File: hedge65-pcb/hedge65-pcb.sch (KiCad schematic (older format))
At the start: 164 parts, among them J1 USB_C_Receptacle_USB2.0, SW1 SW_PUSH, U1 ATmega32U4-AU, Y1 16MHz

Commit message: schematic done
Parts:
- C1, C2, C3, C4, C5, C6, C7: footprint (none) -> Capacitor_SMD:C_0805_2012Metric
- D1, D10, D11, D12, D13, D14, D15, D16, D17, D18, D19, D2, D20, D21, D22, D23, D24, D25, D26, D27, D28, D29, D3, D30, D31, D32, D33, D34, D35, D36, D37, D38, D39, D4, D40, D41, D42, D43, D44, D45, D46, D47, D48, D49, D5, D50, D51, D52, D53, D54, D55, D56, D57, D58, D59, D6, D60, D61, D62, D63, D64, D65, D66, D67, D68, D69, D7, D70, D71, D72, D73, D8, D9: footprint (none) -> Diode_SMD:D_SOD-123
- F1: footprint (none) -> Fuse:Fuse_1206_3216Metric
- J1: footprint (none) -> Type-C:HRO-TYPE-C-31-M-12-HandSoldering
- Y1: footprint (none) -> Crystal:Crystal_SMD_3225-4Pin_3.2x2.5mm

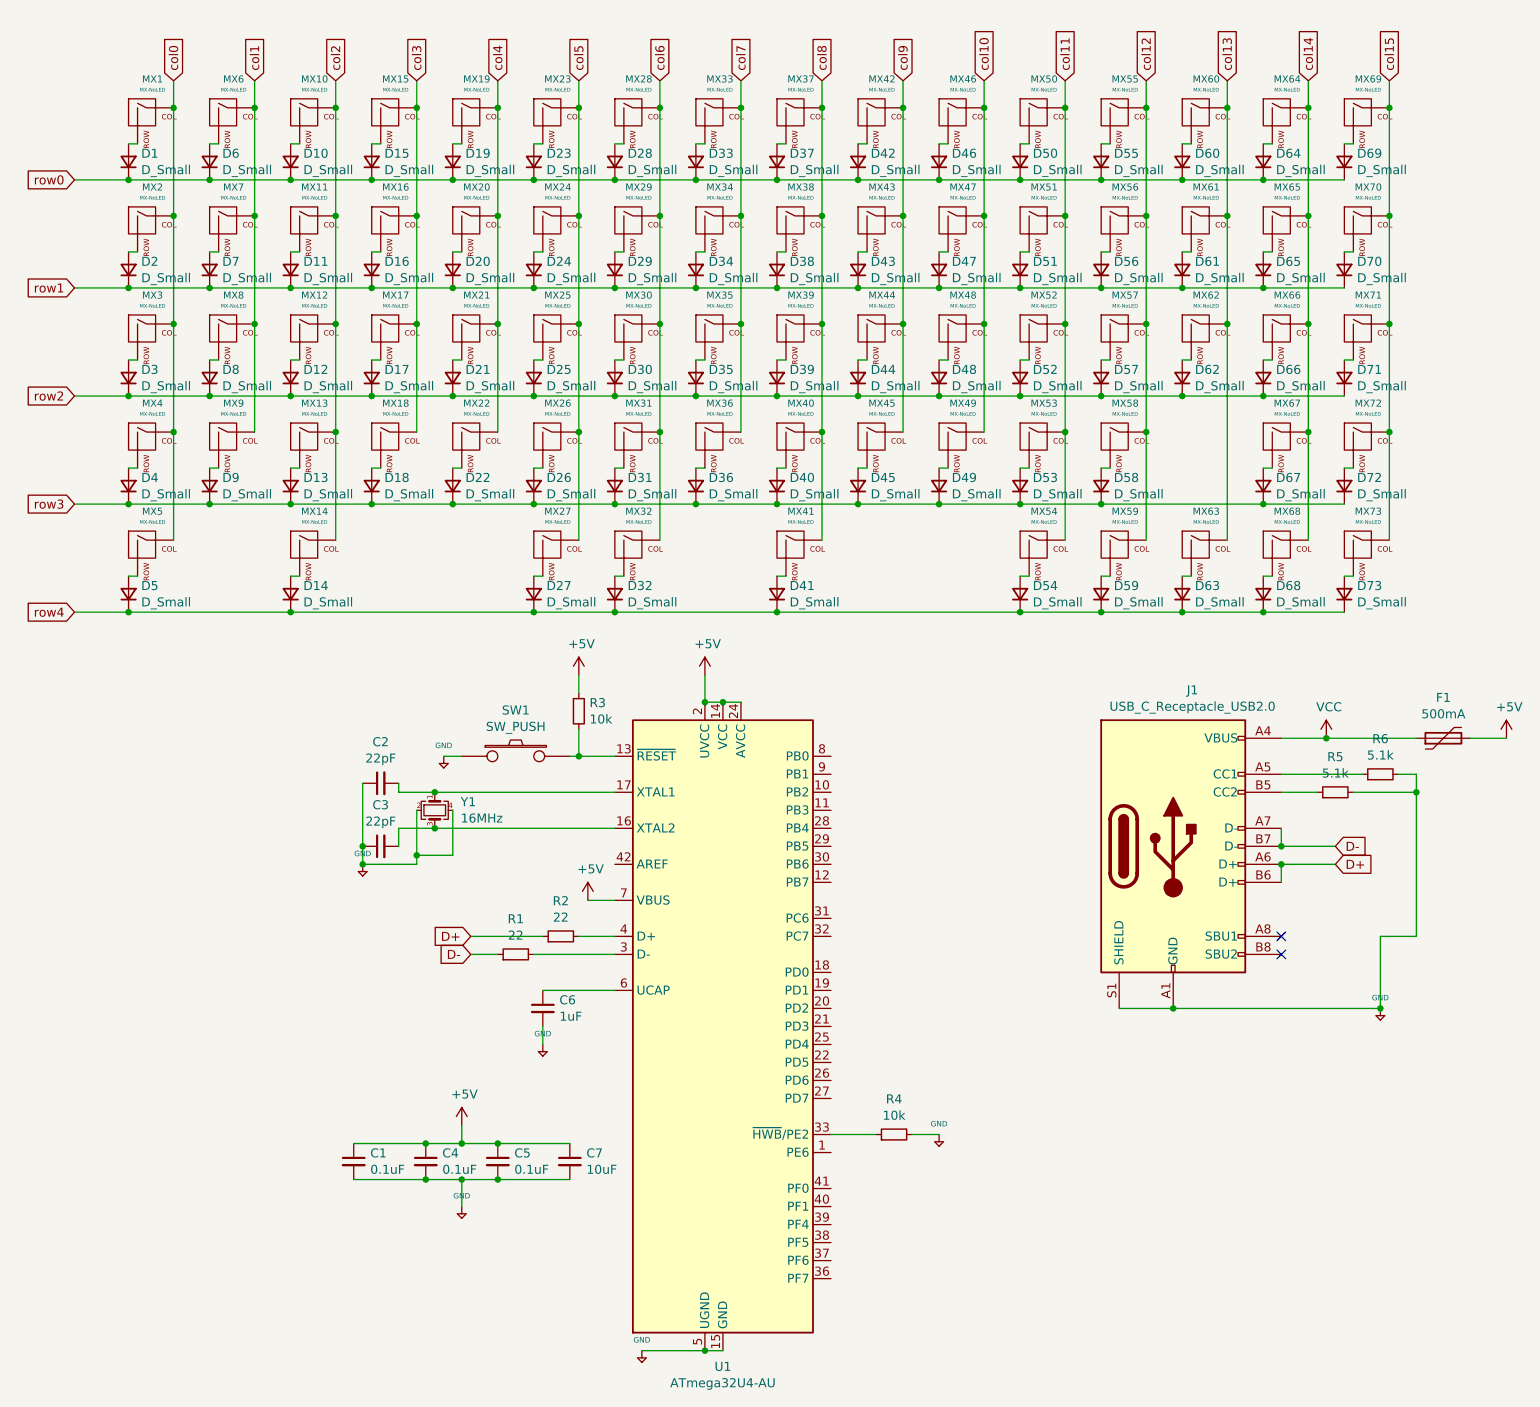
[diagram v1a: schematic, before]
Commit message: redo
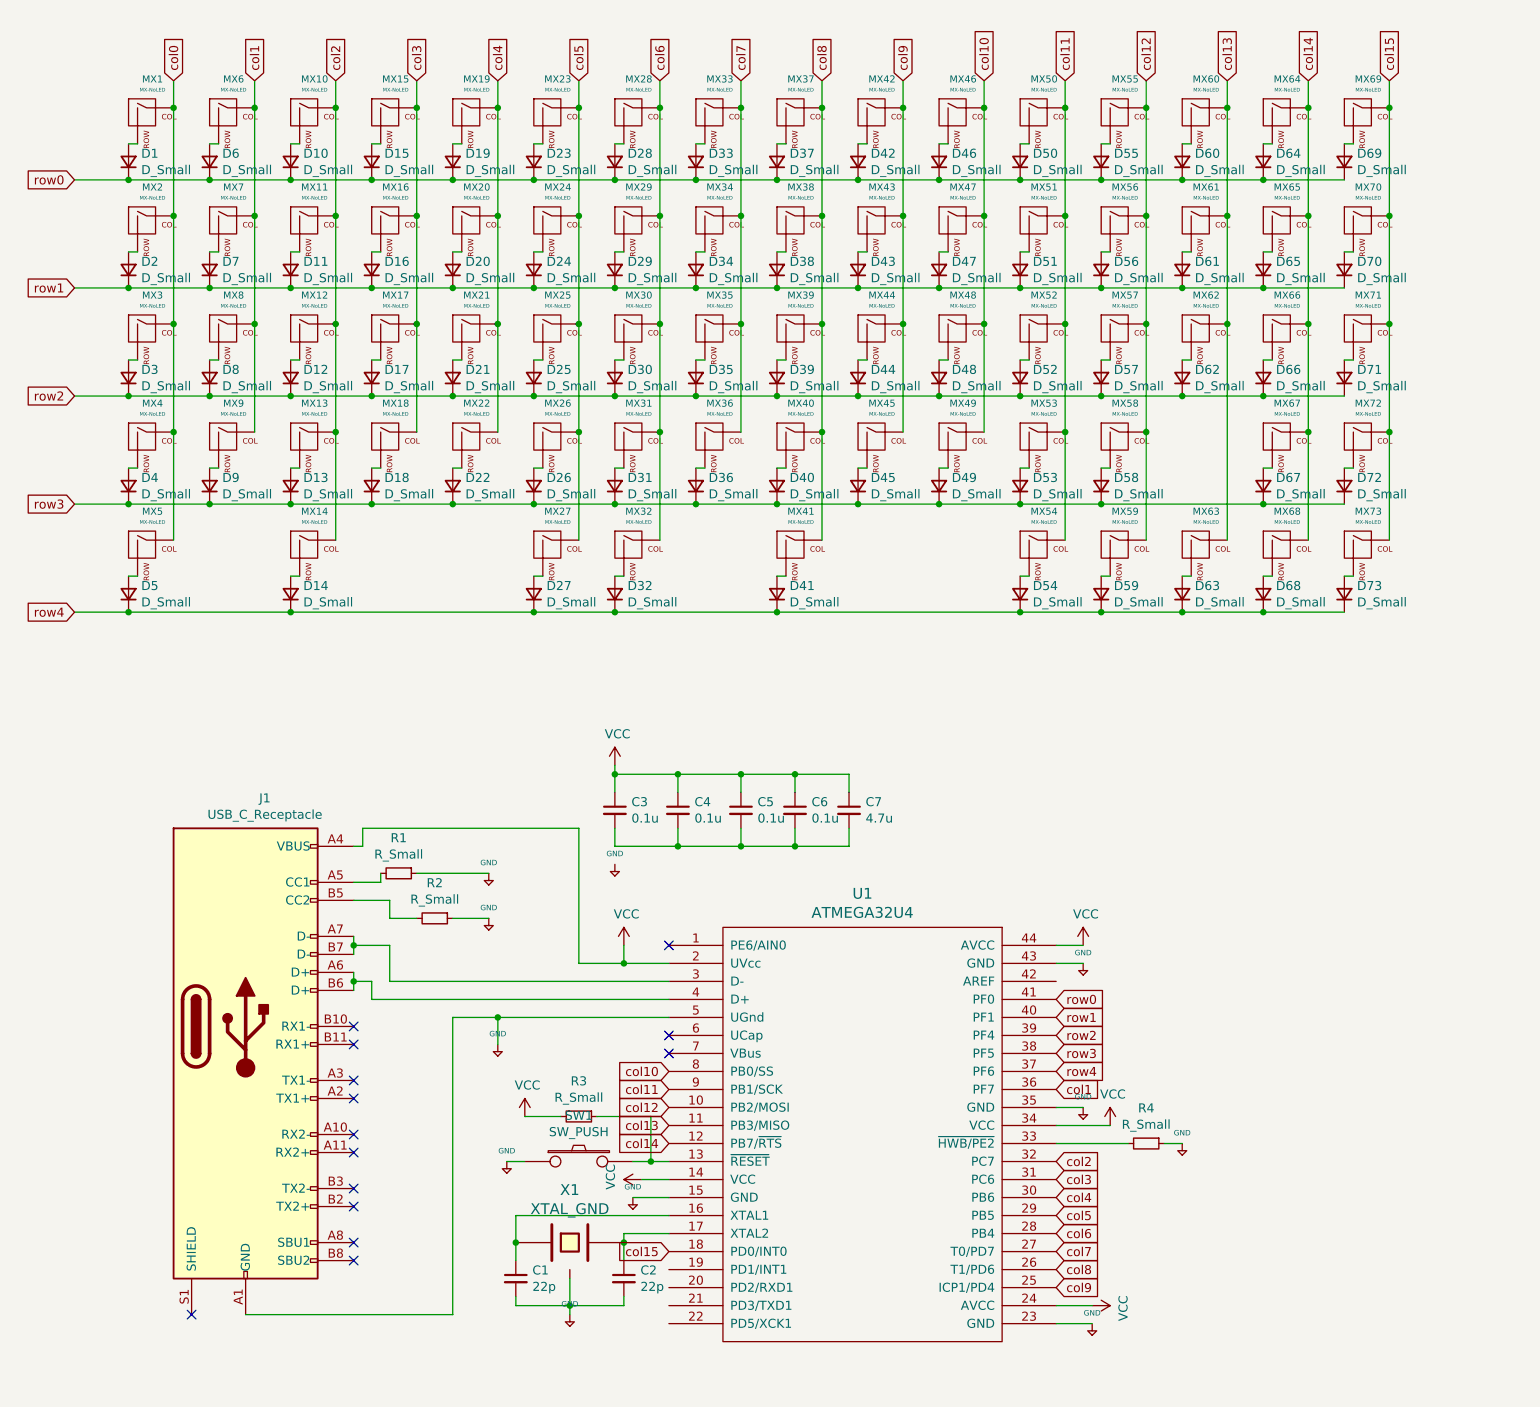
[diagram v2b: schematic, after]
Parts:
- removed F1: 500mA, Fuse:Fuse_1206_3216Metric, symbol Device:Polyfuse
- removed J1: USB_C_Receptacle_USB2.0, Type-C:HRO-TYPE-C-31-M-12-HandSoldering, symbol Connector:USB_C_Receptacle_USB2.0
- removed R5, R6: 5.1k, Resistor_SMD:R_0805_2012Metric, symbol Device:R_Small
- removed U1: ATmega32U4-AU, Package_QFP:TQFP-44_10x10mm_P0.8mm, symbol MCU_Microchip_ATmega:ATmega32U4-AU
- removed Y1: 16MHz, Crystal:Crystal_SMD_3225-4Pin_3.2x2.5mm, symbol Device:Crystal_GND24_Small
- added J1: USB_C_Receptacle, symbol Connector:USB_C_Receptacle
- added U1: ATMEGA32U4, ATmega32U4:ATmega32U4, symbol keyboard_parts:ATMEGA32U4
- added X1: XTAL_GND, Crystal:Crystal_SMD_3225-4Pin_3.2x2.5mm, symbol keyboard_parts:XTAL_GND
- C1: value 0.1uF -> 22p
- C2: value 22pF -> 22p
- C3: value 22pF -> 0.1u
- C4, C5: value 0.1uF -> 0.1u
- C6: value 1uF -> 0.1u
- C7: value 10uF -> 4.7u
- D1, D10, D11, D12, D13, D14, D15, D16, D17, D18, D19, D2, D20, D21, D22, D23, D24, D25, D26, D27, D28, D29, D3, D30, D31, D32, D33, D34, D35, D36, D37, D38, D39, D4, D40, D41, D42, D43, D44, D45, D46, D47, D48, D49, D5, D50, D51, D52, D53, D54, D55, D56, D57, D58, D59, D6, D60, D61, D62, D63, D64, D65, D66, D67, D68, D69, D7, D70, D71, D72, D73, D8, D9: footprint Diode_SMD:D_SOD-123 -> cftkb:D_DO-35_SOD27_P5.08mm_Horizontal
- R1, R2: value 22 -> R_Small
- R3, R4: value 10k -> R_Small
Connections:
- net D+ is gone; now on net +5V: R2.1
- net D- is gone; now on net +5V: R1.1
- net +5V: now also C2.2, R4.1, J1.A1 (GND), J1.A12 (GND), J1.B1 (GND), J1.B12 (GND), U1.15 (GND), U1.23 (GND), U1.35 (GND), U1.43 (GND), U1.5 (UGnd), X1.3; no longer C1.1, C2.1, C3.1, C4.1, C4.2, C5.1, C5.2, C6.2, C7.1, C7.2, R3.1, R4.2
- net VCC: now also C3.1, C4.1, C5.1, C6.1, C7.1, R3.2, J1.A4 (VBUS), J1.A9 (VBUS), J1.B4 (VBUS), J1.B9 (VBUS), U1.14 (VCC), U1.2 (UVcc), U1.24 (AVCC), U1.34 (VCC), U1.44 (AVCC)
- net col1: now also U1.36 (PF7)
- net col10: now also U1.8 (PB0/SS)
- net col11: now also U1.9 (PB1/SCK)
- net col12: now also U1.10 (PB2/MOSI)
- net col13: now also U1.11 (PB3/MISO)
- net col14: now also U1.12 (PB7/~RTS)
- net col15: now also U1.18 (PD0/INT0)
- net col2: now also U1.32 (PC7)
- net col3: now also U1.31 (PC6)
- net col4: now also U1.30 (PB6)
- net col5: now also U1.29 (PB5)
- net col6: now also U1.28 (PB4)
- net col7: now also U1.27 (T0/PD7)
- net col8: now also U1.26 (T1/PD6)
- net col9: now also U1.25 (ICP1/PD4)
- net row0: now also U1.41 (PF0)
- net row1: now also U1.40 (PF1)
- net row2: now also U1.39 (PF4)
- net row3: now also U1.38 (PF5)
- net row4: now also U1.37 (PF6)
- net at SW1.2: now also R3.1, U1.13 (~RESET); no longer R3.2
- net at C3.2: now also C4.2, C5.2, C6.2, C7.2
- net at R1.2: now also J1.A5 (CC1)
- net at R2.2: now also J1.B5 (CC2)
- new net: C1.1, U1.16 (XTAL1), X1.1
- new net: C2.1, U1.17 (XTAL2), X1.2
- new net: J1.A7 (D-), J1.B7 (D-), U1.3 (D-)
- new net: R4.2, U1.33 (~HWB/PE2)
- new net: J1.A6 (D+), J1.B6 (D+), U1.4 (D+)
- no-connect marks 2 -> 14
